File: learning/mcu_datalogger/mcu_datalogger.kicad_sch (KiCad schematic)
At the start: 29 parts, among them J1 Conn_01x09_Pin, J2 Conn_01x04_Pin, J3 Conn_01x04_Pin, J4 Conn_02x03_Odd_Even, U1 24LC1025, U2 DS1337S_, U3 24LC1025, U4 ATMEGA328P-AU, Y1 Crystal, Y2 Crystal

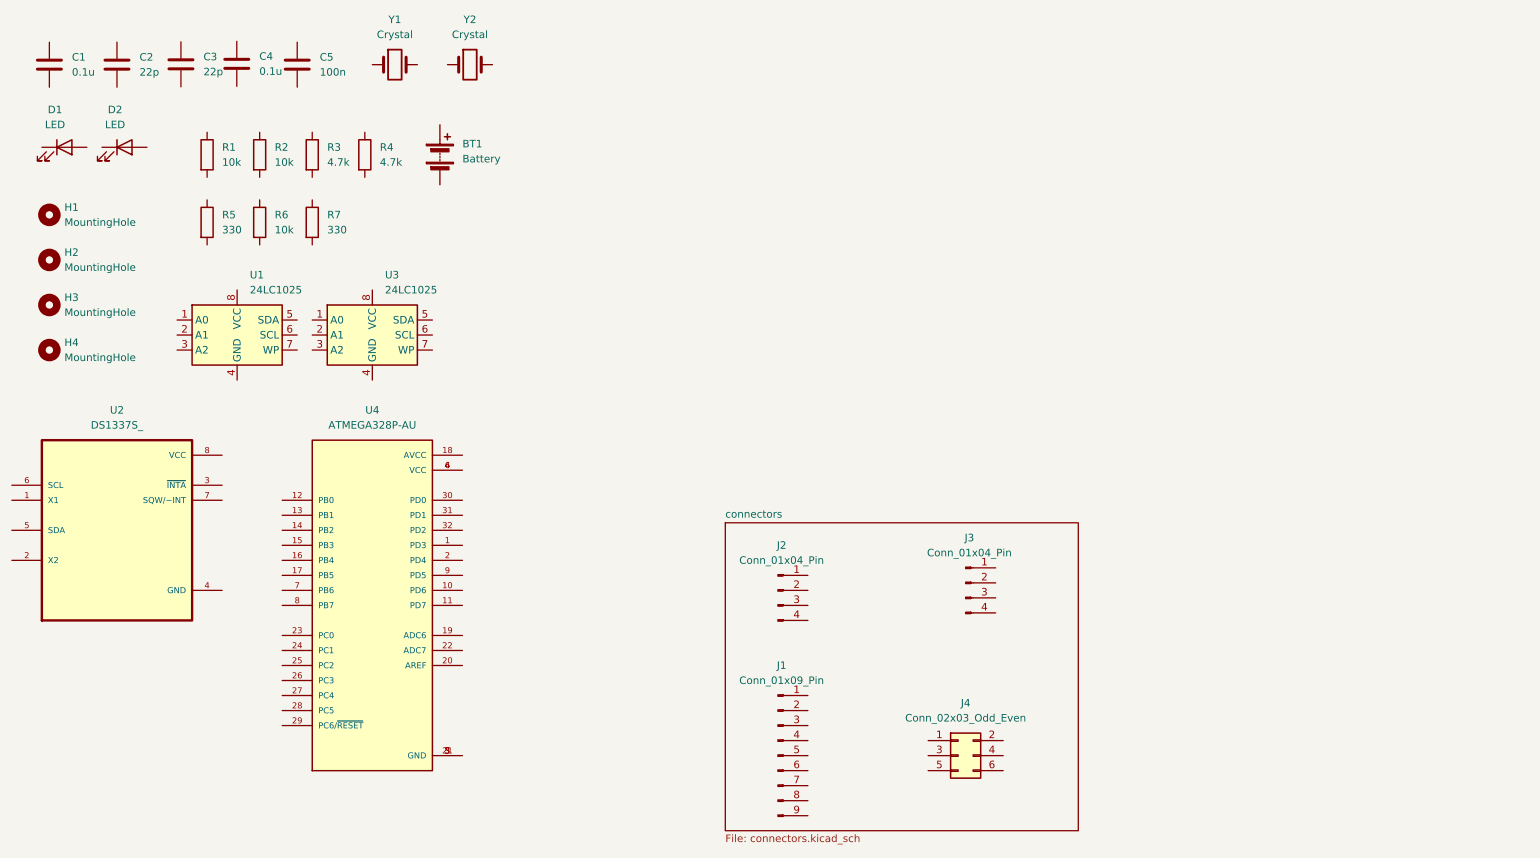
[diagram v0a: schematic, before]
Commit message: Finished the schematic design
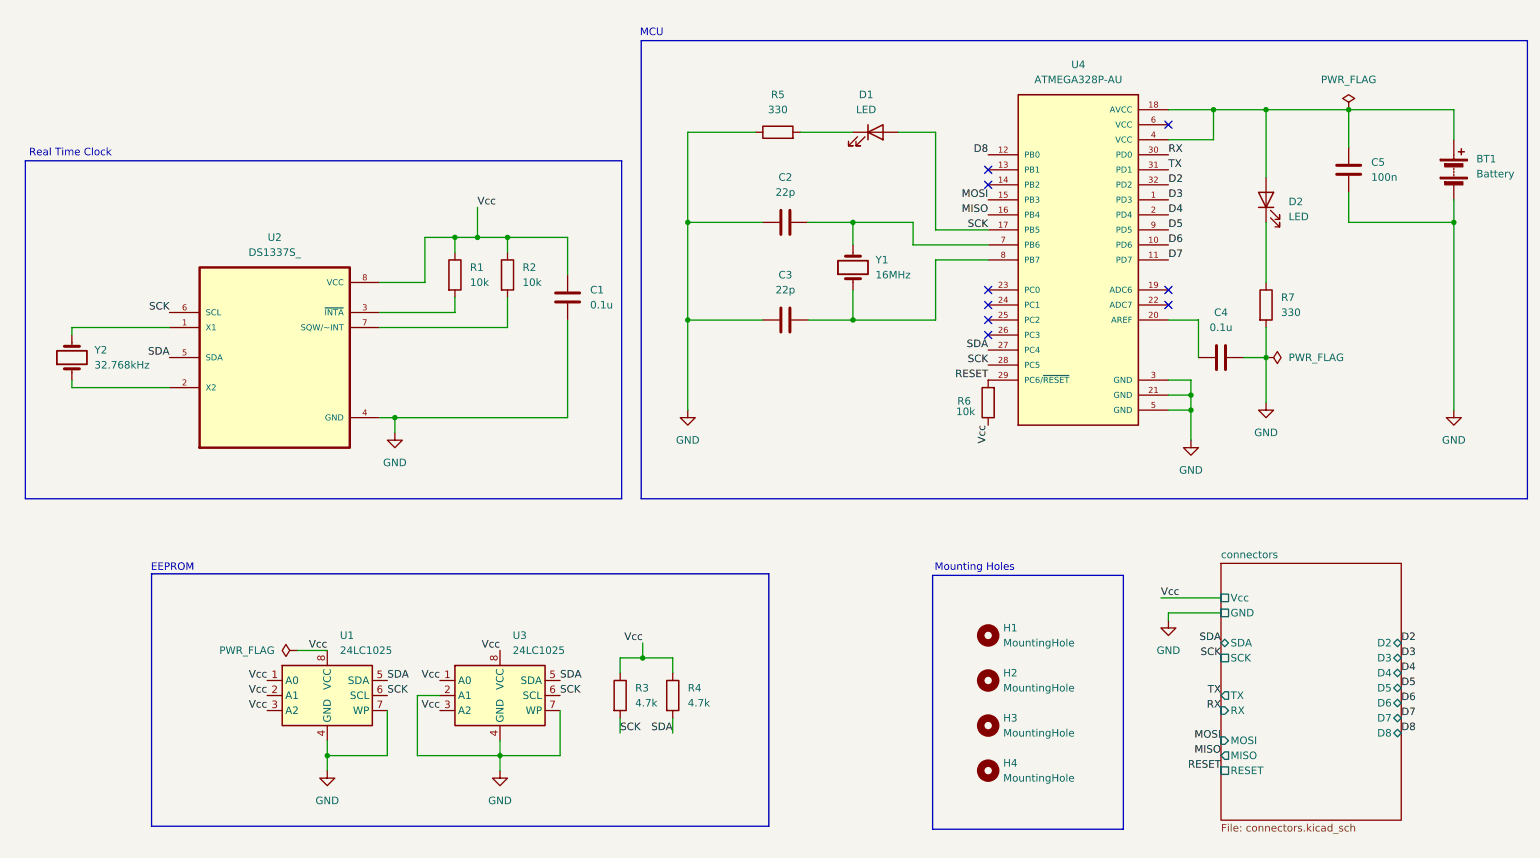
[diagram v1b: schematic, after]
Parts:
- removed J1: Conn_01x09_Pin, symbol Connector:Conn_01x09_Pin
- removed J2, J3: Conn_01x04_Pin, symbol Connector:Conn_01x04_Pin
- removed J4: Conn_02x03_Odd_Even, symbol Connector_Generic:Conn_02x03_Odd_Even
- BT1: footprint (none) -> Connector_PinHeader_2.54mm:PinHeader_1x02_P2.54mm_Vertical
- C1, C2, C3, C4, C5: footprint (none) -> Capacitor_SMD:C_0805_2012Metric
- D1, D2: footprint (none) -> LED_SMD:LED_0805_2012Metric
- H1, H2, H3, H4: footprint (none) -> MountingHole:MountingHole_2.1mm
- R1, R2, R3, R4, R5, R6, R7: footprint (none) -> Resistor_SMD:R_0805_2012Metric
- U1, U3: footprint (none) -> Package_SO:SOIC-8_5.3x5.3mm_P1.27mm
- U4: footprint ATMEGA328P-AU:QFP80P900X900X120-32N -> Atmega328p-au:QFP80P900X900X120-32N
- Y1: value Crystal -> 16MHz; footprint (none) -> Crystal:Crystal_SMD_5032-2Pin_5.0x3.2mm_HandSoldering
- Y2: value Crystal -> 32.768kHz; footprint (none) -> Crystal:Crystal_SMD_5032-2Pin_5.0x3.2mm_HandSoldering
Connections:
- net Vcc: now reaches R2.1
- net Vcc: now also C1.1, R1.1, R3.1, R4.1, R6.1, U1.1 (A0), U1.2 (A1), U1.3 (A2), U1.8 (VCC), U2.8 (VCC), U3.1 (A0), U3.3 (A2), U3.8 (VCC)
- net at R2.2: now also U2.7 (SQW/~INT)
- net at Y2.1: now also U2.2 (X2)
- net at Y2.2: now also U2.1 (X1)
- net at Y1.1: now also C3.2, U4.8 (PB7)
- net at Y1.2: now also C2.2, U4.7 (PB6)
- net at U2.3 (~{INTA}): now also R1.2
- net GND: now reaches U2.4 (GND)
- net GND: now also BT1.2 (-), C1.2, C2.1, C3.1, C4.2, C5.2, R5.1, R7.2, U1.4 (GND), U1.7 (WP), U3.2 (A1), U3.4 (GND), U3.7 (WP), U4.21 (GND), U4.3 (GND), U4.5 (GND)
- net SDA: now reaches U2.5 (SDA)
- net SDA: now also R4.2, U1.5 (SDA), U3.5 (SDA), U4.27 (PC4)
- net SCK: now reaches U2.6 (SCL)
- net SCK: now also D1.2 (A), R3.2, U1.6 (SCL), U3.6 (SCL), U4.17 (PB5), U4.28 (PC5)
- net at D1.1 (K): now also R5.2
- net at C5.1: now also BT1.1 (+), D2.2 (A), U4.18 (AVCC), U4.4 (VCC)
- net at R7.1: now also D2.1 (K)
- net RESET: now reaches R6.2
- net RESET: now also U4.29 (PC6/~{RESET})
- net D3: now reaches U4.1 (PD3)
- net D6: now reaches U4.10 (PD6)
- net D7: now reaches U4.11 (PD7)
- net D8: now reaches U4.12 (PB0)
- net MOSI: now reaches U4.15 (PB3)
- net MISO: now reaches U4.16 (PB4)
- net D4: now reaches U4.2 (PD4)
- net at U4.20 (AREF): now also C4.1
- net RX: now reaches U4.30 (PD0)
- net TX: now reaches U4.31 (PD1)
- net D2: now reaches U4.32 (PD2)
- net at U4.6 (VCC): no longer U4.4 (VCC)
- net D5: now reaches U4.9 (PD5)
- no-connect marks 0 -> 9
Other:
- sheet connectors ports: added D2, D3, D4, D5, D6, D7, D8, GND, MISO, MOSI, RESET, RX, SCK, SDA, TX, Vcc; removed none
- note added: "EEPROM"
- note added: "MCU"
- note added: "Mounting Holes"
- note added: "Real Time Clock"
- moved on the sheet: BT1, C1, C2, C3, C4, C5, D1, D2, H1, H2, H3, H4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
